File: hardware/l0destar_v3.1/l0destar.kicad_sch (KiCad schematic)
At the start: 9 parts

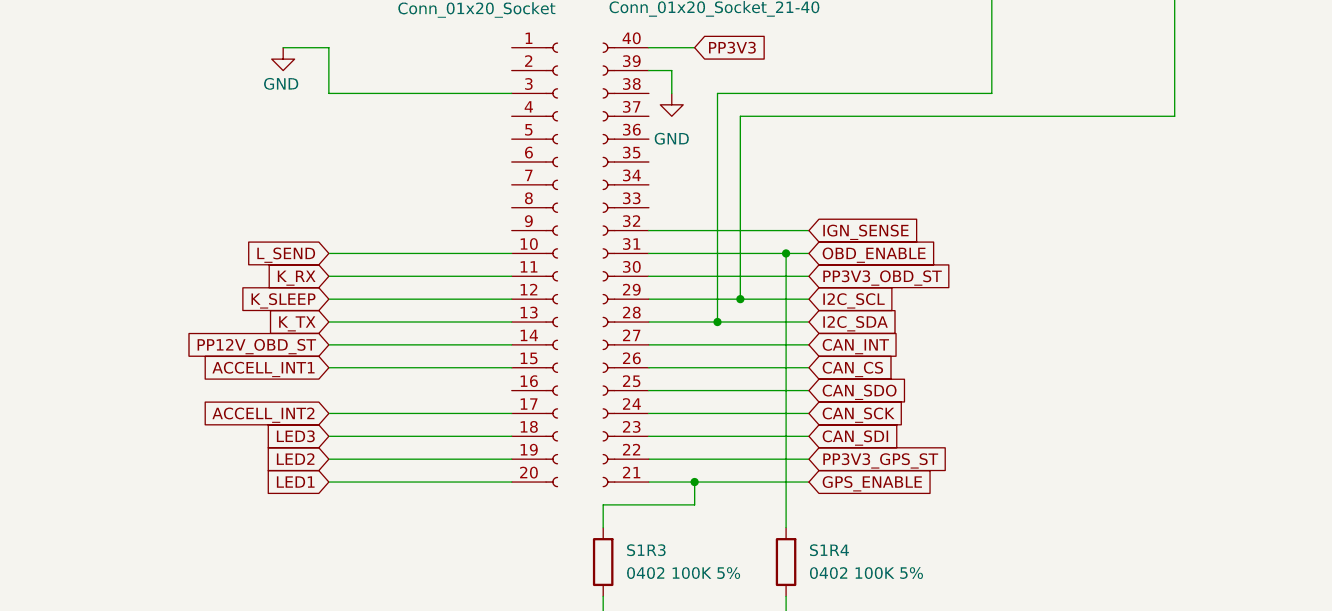
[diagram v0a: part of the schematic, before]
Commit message: update v3.1
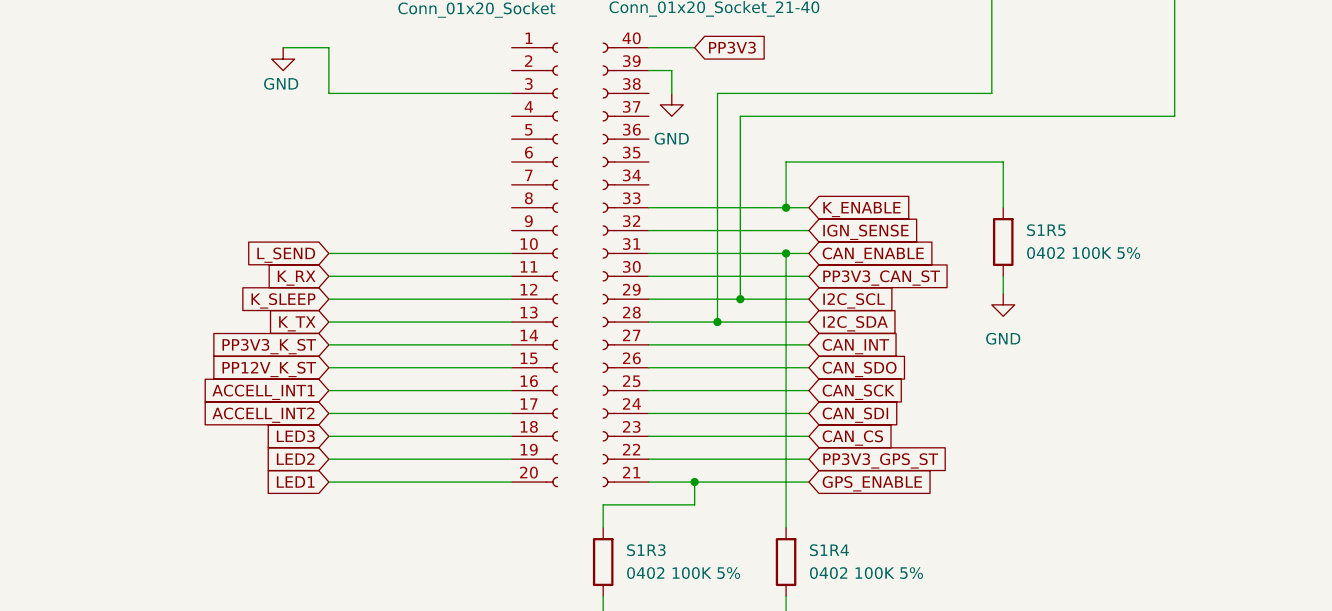
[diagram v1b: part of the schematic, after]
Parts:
- added S1R5: 0402 100K 5%, Resistor_SMD:R_0402_1005Metric, symbol Device:R
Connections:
- net ACCELL_INT1: now also S1J2.16 (Pin_16); no longer S1J2.15 (Pin_15)
- net CAN_CS: now also S1J3.23 (Pin_18); no longer S1J3.26 (Pin_15)
- net CAN_SCK: now also S1J3.25 (Pin_16); no longer S1J3.24 (Pin_17)
- net CAN_SDI: now also S1J3.24 (Pin_17); no longer S1J3.23 (Pin_18)
- net CAN_SDO: now also S1J3.26 (Pin_15); no longer S1J3.25 (Pin_16)
- net GND: now also S1R5.1
- net K_ENABLE: now reaches S1J3.33 (Pin_8)
- net K_ENABLE: now also S1R5.2
- net OBD_ENABLE renamed CAN_ENABLE
- net PP12V_OBD_ST renamed PP3V3_K_ST
- net PP3V3_OBD_ST renamed PP3V3_CAN_ST
- new net PP12V_K_ST: S1J2.15 (Pin_15)
